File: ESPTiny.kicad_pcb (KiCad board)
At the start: 2 copper layers, 33 x 26.4 mm, 21 parts, among them J1 Conn_01x10_Male, J2 Conn_01x10_Male, J3 Conn_01x04_Male, U1 ESP-01v090, U2 ATtiny84-20PU, U3 MCP1700-3302E_TO92

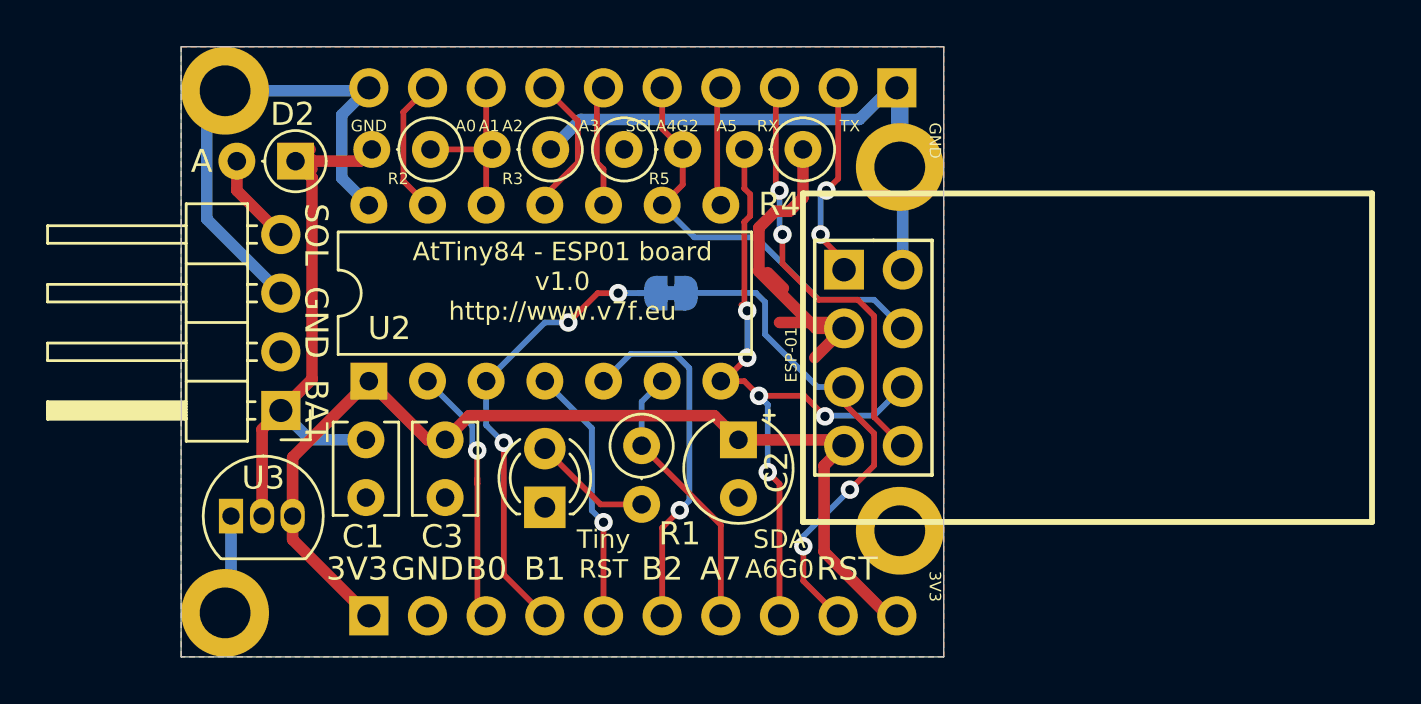
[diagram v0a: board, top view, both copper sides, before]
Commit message: 1.1 repositioning
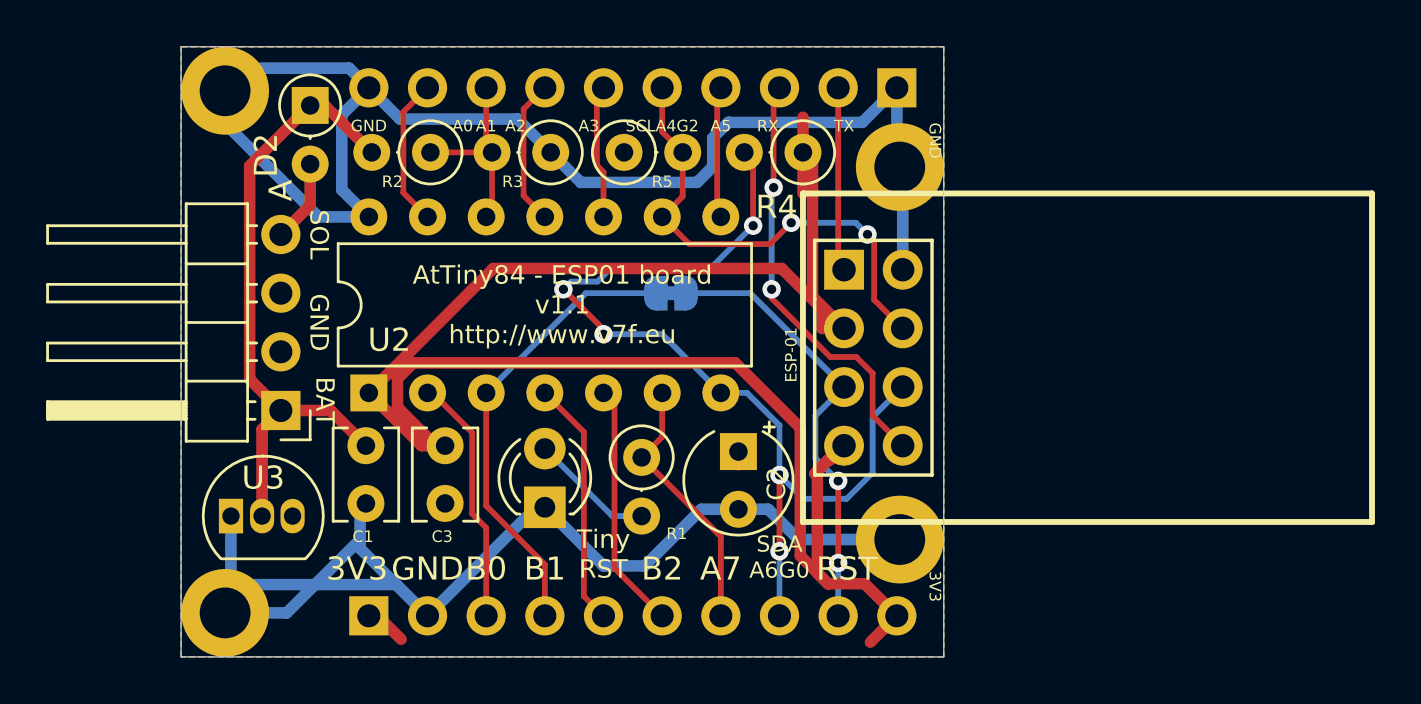
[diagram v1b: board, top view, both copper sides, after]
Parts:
- moved D2 2.50 mm to (44.7, 42.9), turned to 270 degrees
- moved U2 0.51 mm to (47.2, 55.4)
- moved C2 0.51 mm to (63.2, 57.9)
- moved R1 0.51 mm to (59.1, 58.2)
- moved REF** 0.38 mm to (70.2, 61.7)
- moved C1 0.25 mm to (47.1, 57.7)
- moved C3 0.25 mm to (50.5, 57.7)
- moved R2 0.13 mm to (49.9, 45.0)
- moved R3 0.13 mm to (55.1, 45.0)
- moved R4 0.13 mm to (66.0, 45.0)
- moved R5 0.13 mm to (58.3, 45.0)
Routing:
- net GND: track 54.8 -> 111.0 mm
- net +3V3: track 61.9 -> 87.2 mm
- net /SDA-A6: track 30.4 -> 43.6 mm
- net /B2: track 15.7 -> 10.7 mm, vias 1 -> 0
- net /SCL-A4: track 18.4 -> 21.6 mm, vias 0 -> 2
- net /RST: track 22.0 -> 19.4 mm
- net +BATT: track 25.9 -> 27.6 mm
- net /B1: track 21.4 -> 19.8 mm, vias 3 -> 0
- net /TRST: track 11.9 -> 10.7 mm, vias 1 -> 0
- net Net-(D2-Pad2): track 4.68 -> 3.57 mm
- net /TX: track 9.02 -> 7.98 mm, vias 2 -> 0
- net /B0: track 11.4 -> 10.8 mm, vias 1 -> 0
- net /A1: track 7.96 -> 8.47 mm
- net /A3: track 5.32 -> 5.82 mm
- net /A0: track 5.95 -> 6.46 mm
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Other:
- board text added: "AtTiny84 - ESP01 board v1.1 http://www.v7f.eu"
- board text removed: "AtTiny84 - ESP01 board v1.0 http://www.v7f.eu"
